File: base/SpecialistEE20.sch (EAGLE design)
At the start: 105 parts, among them X1 SCART-F

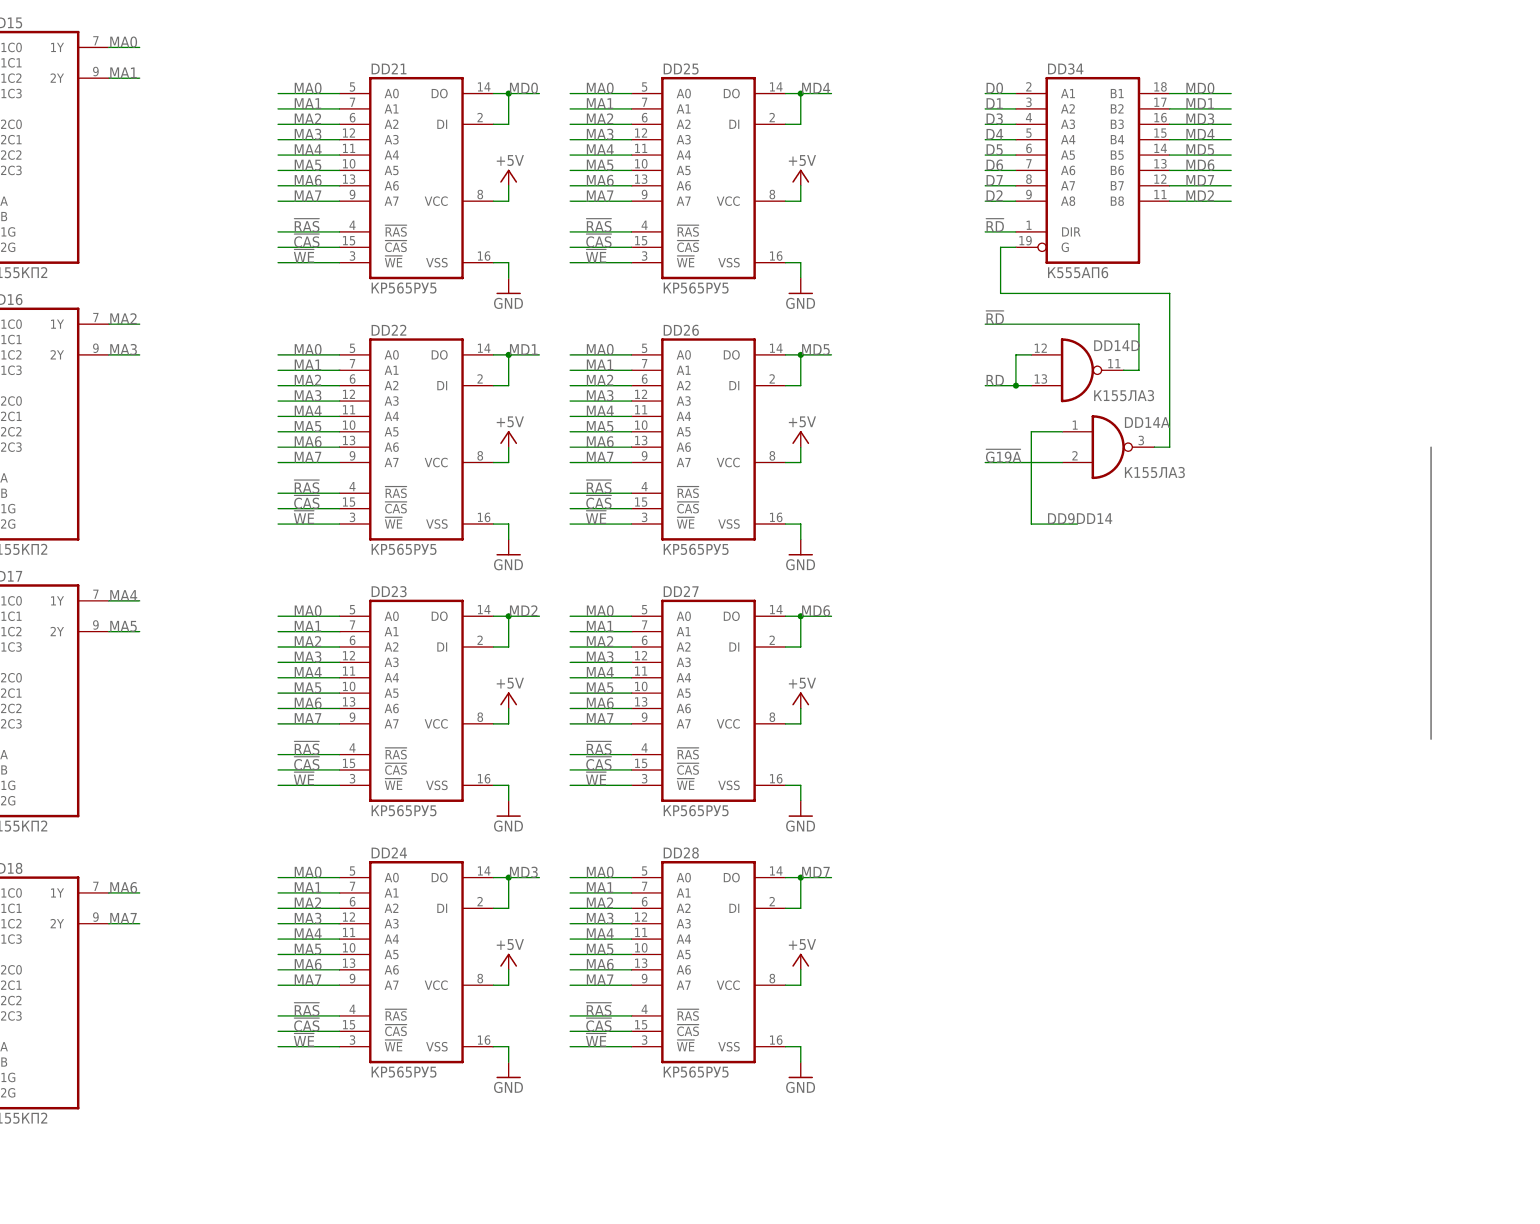
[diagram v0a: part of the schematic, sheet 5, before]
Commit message: .
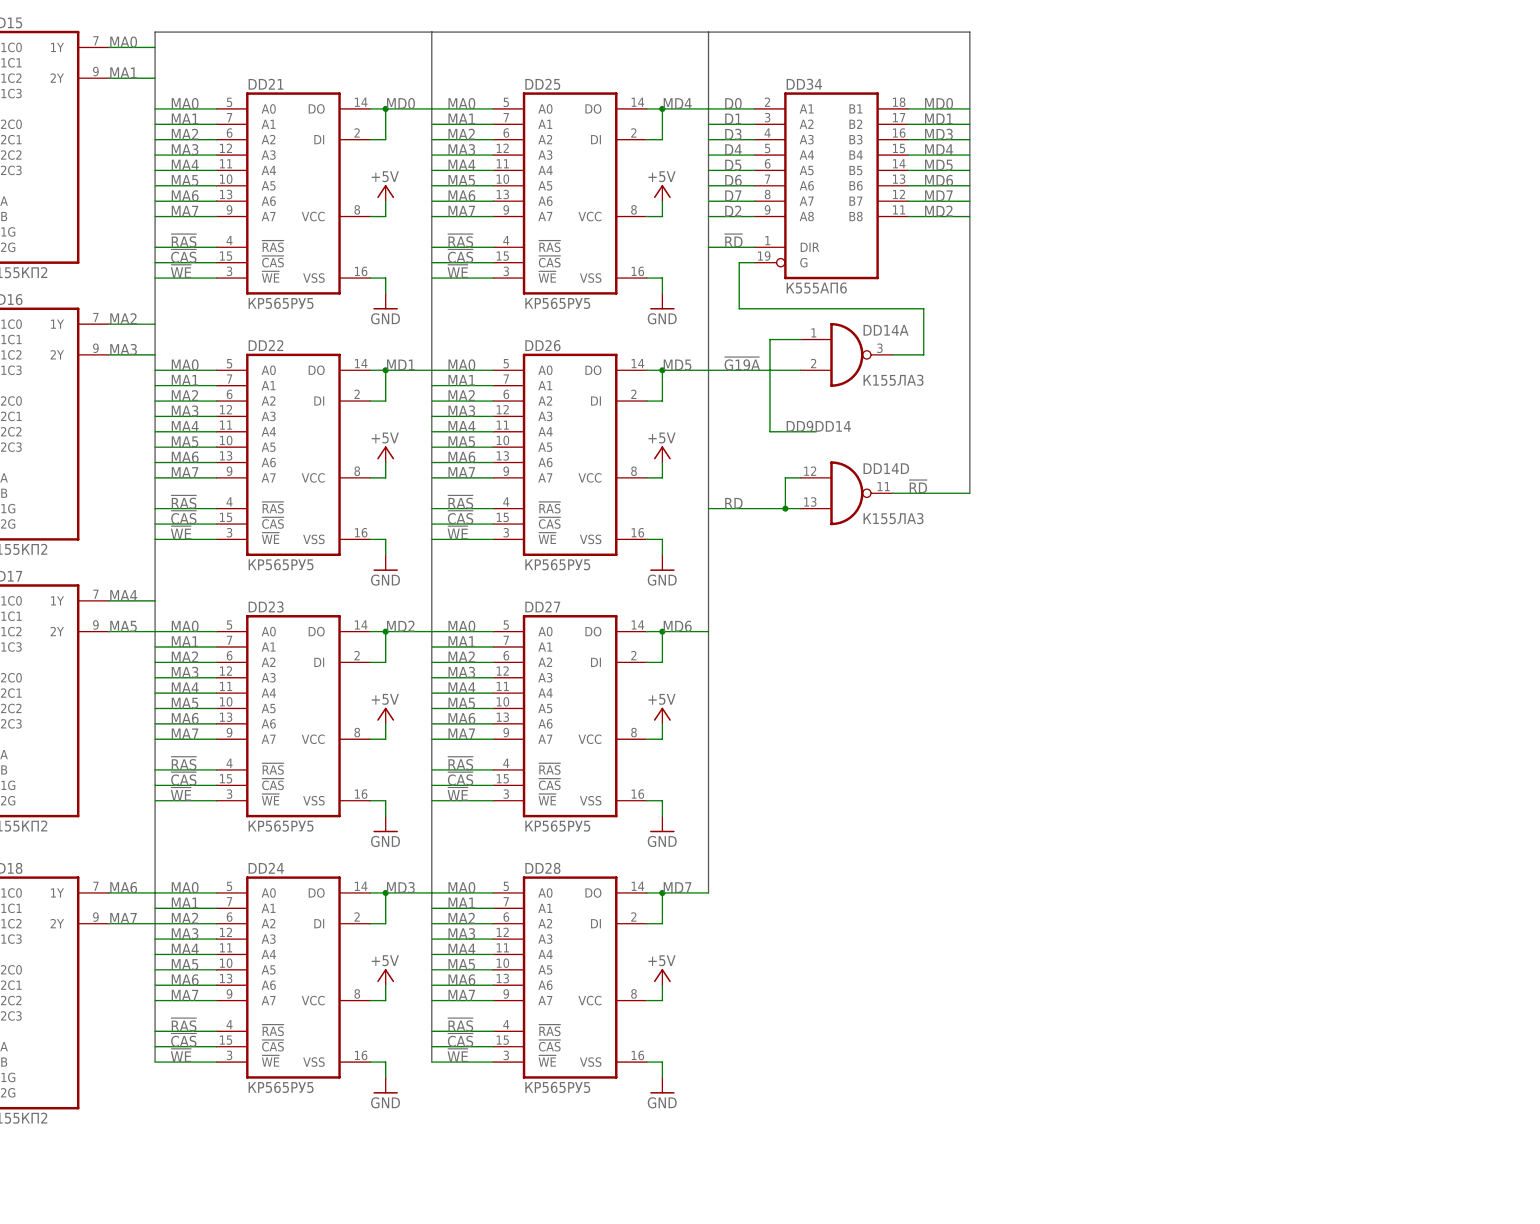
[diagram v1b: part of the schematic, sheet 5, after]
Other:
- moved on the sheet: DD14A, DD14D, DD21, DD22, DD23, DD24, DD25, DD26, DD27, DD28, DD34
